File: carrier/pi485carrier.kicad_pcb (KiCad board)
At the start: 2 copper layers, 62.9 x 29.8 mm, 21 parts, among them P1 PWR, P2 Rasperry Pi, P3 Latch Disable, P4 TERM, P5 CONN_01X04, P6 CONN_01X04, Q1 2N4401, Q2 2N4401, Q3 2N4401, U1 NE555

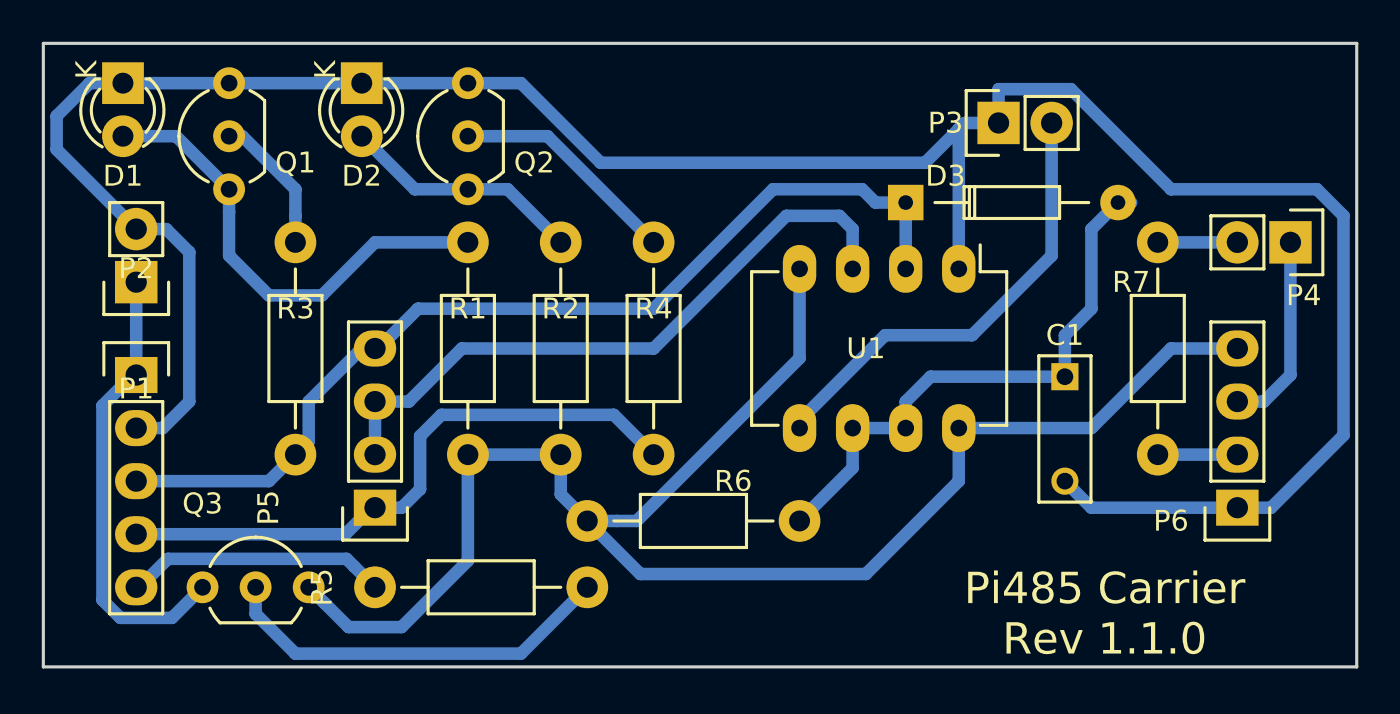
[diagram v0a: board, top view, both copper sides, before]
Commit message: Carrier updates.
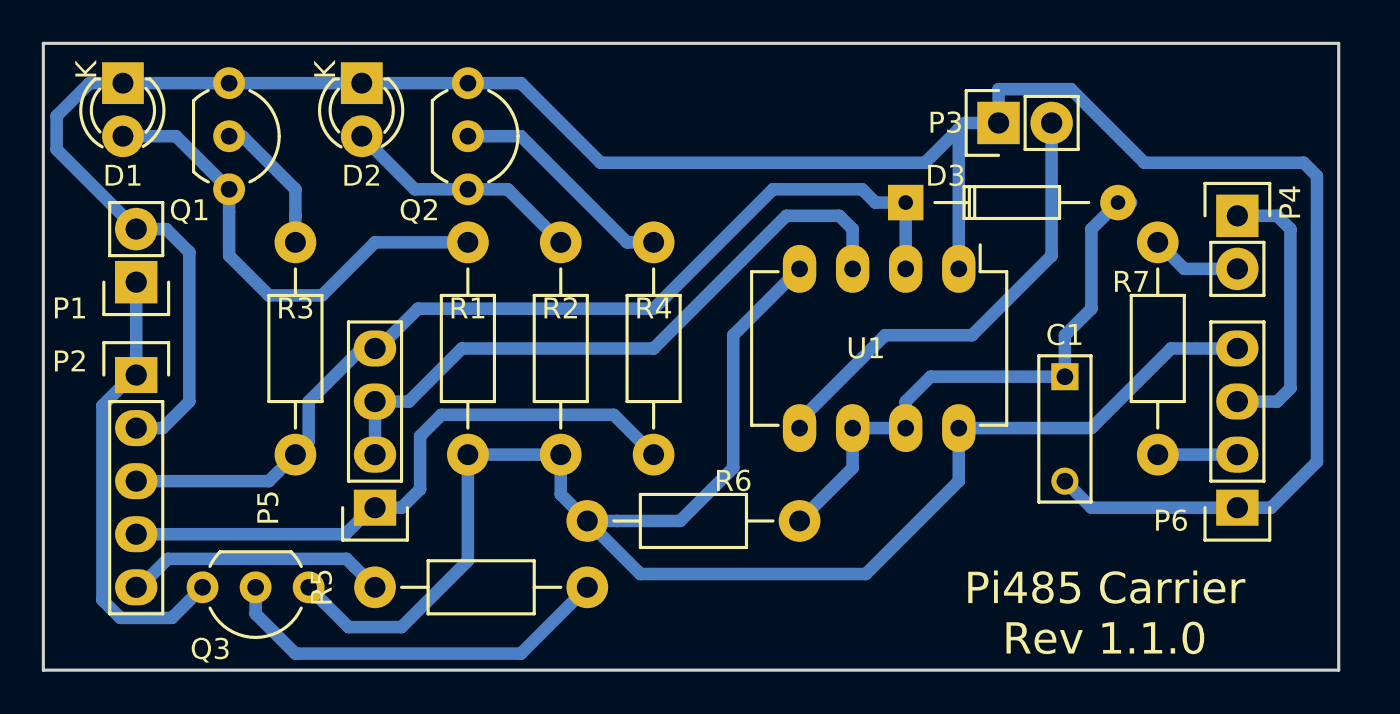
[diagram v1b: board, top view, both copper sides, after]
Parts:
- moved Q1 5.08 mm to (46.4, 22.9), turned to 270 degrees
- moved Q2 5.08 mm to (57.8, 22.9), turned to 270 degrees
- moved Q3 5.08 mm to (50.2, 47.0), turned to 180 degrees
- moved P4 2.84 mm to (94.6, 29.2), turned to 0 degrees
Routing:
- net /lctec485/B: track 9.42 -> 13.2 mm
- net /lctec485/VCIN: track 78.7 -> 80.0 mm
- net GND: track 121.9 -> 121.2 mm
- net Net-(P4-Pad2): track 3.81 -> 4.34 mm
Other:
- board size 62.9 x 29.8 mm -> 62 x 30 mm
